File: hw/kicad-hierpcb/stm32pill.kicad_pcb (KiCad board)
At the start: 2 copper layers, 23.8 x 49 mm, 54 parts, among them SW1 Tactile Switch, SW2 Tactile Switch, U1 3.3V Voltage Regulator 200mA, X1 Crystal 12MHz X322512MSB4SI

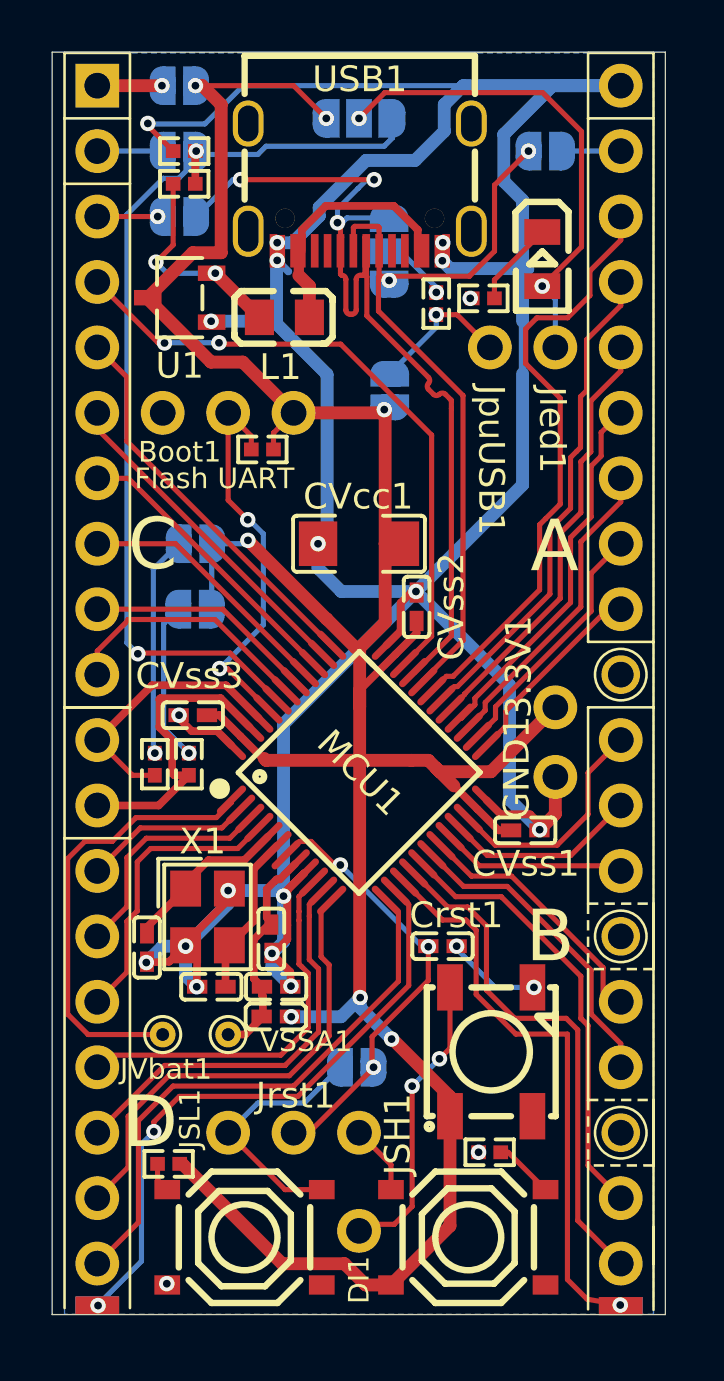
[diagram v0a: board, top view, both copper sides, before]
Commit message: improved layout
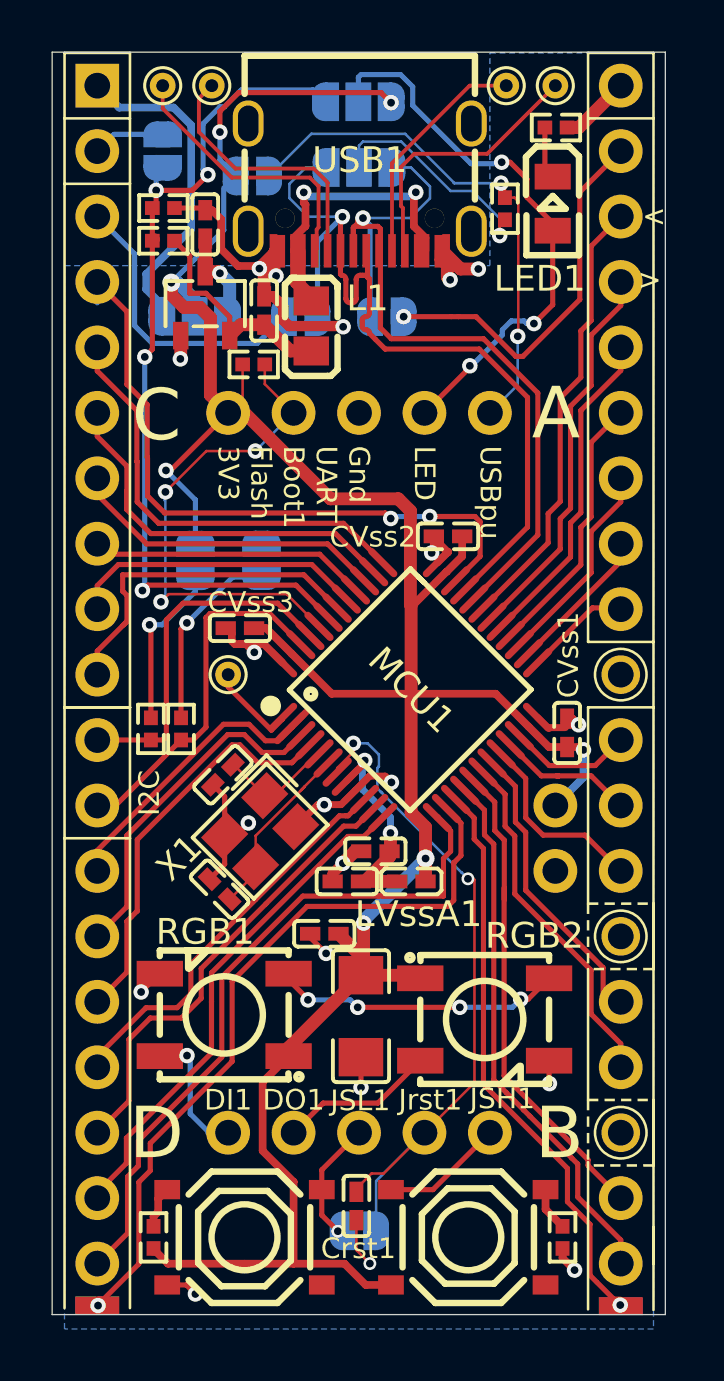
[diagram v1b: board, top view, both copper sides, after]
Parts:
- removed VSSA1: VSSA, TestPoint:TestPoint_THTPad_D1.0mm_Drill0.5mm
- added CC1_1: ~, base:TestPoint_THTPad_D1.0mm_Drill0.5mm, F.Cu at (41.3, 25.4)
- added CC2_1: ~, base:TestPoint_THTPad_D1.0mm_Drill0.5mm, F.Cu at (27.9, 25.4)
- added CLed1: 100nF, jlcpcb:C0402, F.Cu at (34.2, 58.3)
- added CUin1: 1μF, jlcpcb:C0402, F.Cu at (31.9, 34.1)
- added CUout1: 1μF, jlcpcb:C0402, F.Cu at (29.6, 30.8)
- added DO1: ~, base:PTH 1.7mm, F.Cu at (33.0, 66.0)
- added RGB2: LED WS2812B, jlcpcb:LED-SMD_4P-L5.0-W5.0-TL-1, F.Cu at (40.4, 61.6)
- added SBU1_1: ~, base:TestPoint_THTPad_D1.0mm_Drill0.5mm, F.Cu at (29.8, 25.4)
- added SBU2_1: ~, base:TestPoint_THTPad_D1.0mm_Drill0.5mm, F.Cu at (43.2, 25.4)
- JPV1: value SolderJumper_2_Open -> SolderJumper_3_Open; footprint Jumper:SolderJumper-2_P1.3mm_Open_RoundedPad1.0x1.5mm -> Jumper:SolderJumper-3_P1.3mm_Open_RoundedPad1.0x1.5mm
- JVbat1: footprint TestPoint:TestPoint_THTPad_D1.0mm_Drill0.5mm -> base:TestPoint_THTPad_D1.0mm_Drill0.5mm
- RGB1: value LED WS2812B-S XL-5050RGBC -> LED WS2812B
- moved CVcc1 18.3 mm to (35.6, 61.5), turned to -90 degrees
- moved JVbat1 14.2 mm to (30.5, 48.3)
- moved CVss2 11.8 mm to (39.0, 42.9), turned to 0 degrees
- moved Crst1 10.6 mm to (35.5, 68.9), turned to 90 degrees
- moved RGB1 10.5 mm to (30.3, 61.5), turned to 180 degrees
- moved JPpuUSBconst1 9.89 mm to (31.4, 28.9), turned to 180 degrees
- moved JPV1 8.97 mm to (29.2, 34.4), turned to 180 degrees
- moved JPdn1 8.89 mm to (36.6, 34.4)
- moved CVss1 7.62 mm to (43.6, 50.5)
- moved Boot1 7.62 mm to (35.6, 38.1), turned to 180 degrees
- moved LVssA1 7.43 mm to (37.6, 56.3)
- moved Cosc1 7.32 mm to (30.3, 52.1), turned to 45 degrees
- moved Rled1 7.20 mm to (43.2, 27.0), turned to 180 degrees
- moved JPReset1 6.35 mm to (35.6, 69.8)
- moved DI1 6.35 mm to (30.5, 66.0)
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- renumbered CVss2 to CVss1, CVss1 to CVss2
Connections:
- CVcc1 pad 1: GND -> +3.3V
- CVcc1 pad 2: +3.3V -> GND
- IDE_STM_D1 pad SCL: /I2C1 SDA -> /I2C1 SCL
- IDE_STM_D1 pad SDA: /I2C1 SCL -> /I2C1 SDA
- JPV1 pad 1: Net-(IDE_STM_C1-IDE1_STM23) -> Net-(JPV1-A)
- RGB1 pad 2: unconnected-(RGB1-DO-Pad2) -> Net-(RGB1-DO)
- U1 pad 3: +3.3V -> Net-(JPV1-A)
- USB1 pad A5: unconnected-(USB1-CC1-PadA5) -> /CC1
- USB1 pad A8: unconnected-(USB1-SBU1-PadA8) -> /SBU1
- USB1 pad B5: unconnected-(USB1-CC2-PadB5) -> /CC2
- USB1 pad B8: unconnected-(USB1-SBU2-PadB8) -> /SBU2
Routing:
- net GND: track 147.3 -> 45.8 mm, vias 22 -> 20
- net Net-(JPpuUSBconst1-A): track 5.65 -> 20.4 mm, vias 1 -> 2
- net /VBAT: track 17.4 -> 3.52 mm
- net Net-(IDE_STM_A1-IDE4_STM22): track 2.57 -> 14.8 mm, vias 0 -> 1
- net /NRST: track 17.2 -> 29.4 mm, vias 3 -> 2
- net Net-(RGB1-DO): track 0.00 -> 11.3 mm, vias 0 -> 4
- net /CC2: track 0.00 -> 10.7 mm
- net /SBU2: track 0.00 -> 10.6 mm
- net /SBU1: track 0.00 -> 10.5 mm
- net Net-(IDE_STM_C1-IDE1_STM23): track 2.51 -> 12.2 mm, vias 1 -> 0
- net /CC1: track 0.00 -> 9.08 mm
- net Net-(IDE_STM_C1-IDE5_STM25): track 2.54 -> 11.4 mm, vias 1 -> 0
- net /USBd+: track 40.1 -> 33.5 mm, vias 3 -> 1
- net Net-(DI1-Pin_1): track 11.6 -> 5.15 mm, vias 2 -> 1
- net Net-(JPpuUSB1-C): track 2.61 -> 8.97 mm
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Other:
- board text added: "3V3"
- board text added: ">"
- board text added: "Flash"
- board text added: "Gnd"
- board text added: "I2C"
- board text added: "LED"
- board text added: "RX"
- board text added: "Resetswitch"
- board text added: "TX"
- board text added: "UART"
- board text added: "USB"
- board text added: "USBpu"
- board text added: "Vcc"
- board text removed: "Flash UART"
- board text removed: "TX RX"
